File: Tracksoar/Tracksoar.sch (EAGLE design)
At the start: 35 parts, among them IC2 74AHC1G125DBV, U1 ATMEGA328P, Y1 16MHZ

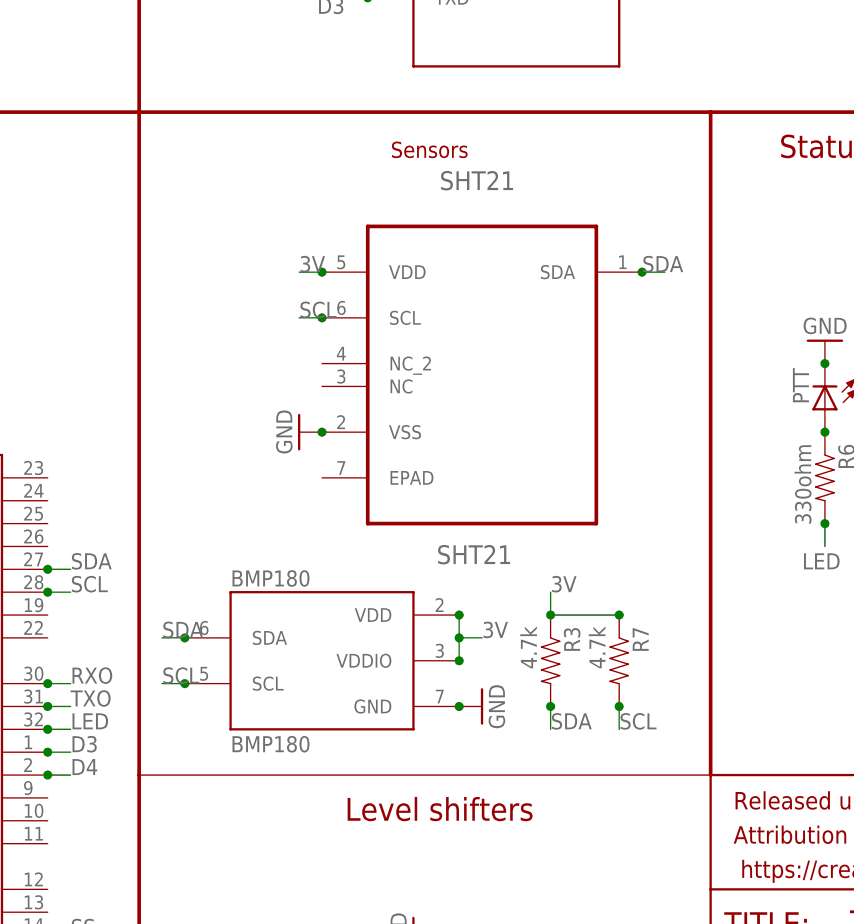
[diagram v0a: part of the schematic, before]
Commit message: Added V1.2 board
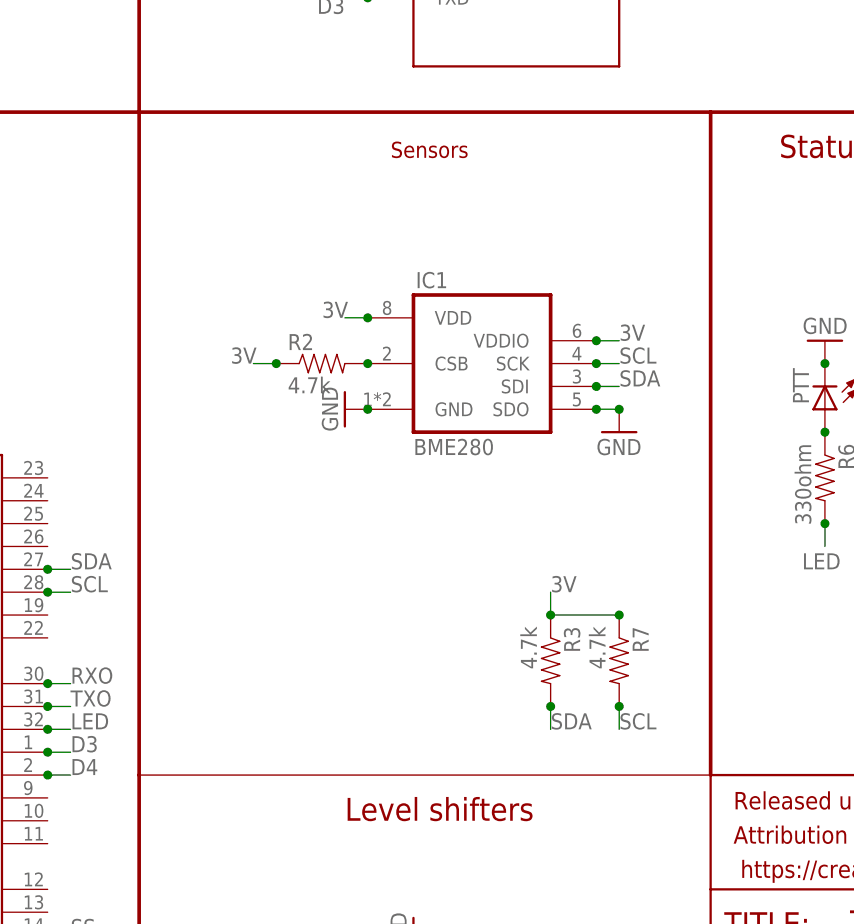
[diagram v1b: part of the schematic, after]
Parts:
- removed BMP180: BMP180, SparkFun-Sensors:BMP180
- removed SHT21: SHT21, sht21:SHT21
- added IC1: BME280, bosch-bme280:BME280
- added R2: 4.7k, SparkFun-Resistors:RESISTOR0805-RES
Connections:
- new net N$2: IC1.CSB, R2.2
- net 3V: now also IC1.VDD, IC1.VDDIO, R2.1; no longer BMP180.VDD, BMP180.VDDIO, SHT21.VDD
- net GND: now also IC1.GND, IC1.SDO; no longer BMP180.GND, SHT21.VSS
- net SCL: now also IC1.SCK; no longer BMP180.SCL, SHT21.SCL
- net SDA: now also IC1.SDI; no longer BMP180.SDA, SHT21.SDA
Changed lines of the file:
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@@
 <part name="GND3" library="SparkFun-Aesthetics" deviceset="GND" device=""/>
 <part name="GND10" library="SparkFun-Aesthetics" deviceset="GND" device=""/>
-<part name="BMP180" library="SparkFun-Sensors" deviceset="BMP180" device=""/>
-<part name="GND16" library="SparkFun-Aesthetics" deviceset="GND" device=""/>
 <part name="GND20" library="SparkFun-Aesthetics" deviceset="GND" device=""/>
 <part name="R3" library="SparkFun-Resistors" deviceset="RESISTOR" device="0805-RES" value="4.7k"/>
@@
 <part name="GND29" library="SparkFun-Aesthetics" deviceset="GND" device=""/>
 <part name="GND30" library="SparkFun-Aesthetics" deviceset="GND" device=""/>
-<part name="SHT21" library="sht21" deviceset="SHT21" device=""/>
 <part name="GPS-ANT" library="SparkFun-RF" deviceset="ANTENNA2" device="SMD3"/>
 <part name="FTDI" library="headers(2mm)" deviceset="1X7" device=""/>
@@
 <part name="U$3" library="headers(2mm)" deviceset="1X2" device=""/>
 <part name="GND5" library="SparkFun-Aesthetics" deviceset="GND" device=""/>
+<part name="IC1" library="bosch-bme280" deviceset="BME280" device=""/>
+<part name="GND6" library="SparkFun-Aesthetics" deviceset="GND" device=""/>
+<part name="R2" library="SparkFun-Resistors" deviceset="RESISTOR" device="0805-RES" value="4.7k"/>
 </parts>
 <sheets>
@@
 <instance part="GND3" gate="1" x="17.78" y="157.48"/>
 <instance part="GND10" gate="1" x="208.28" y="58.42" rot="R90"/>
-<instance part="BMP180" gate="G$1" x="104.14" y="48.26"/>
-<instance part="GND16" gate="1" x="121.92" y="43.18" rot="R90"/>
-<instance part="GND20" gate="1" x="101.6" y="73.66" rot="R270"/>
+<instance part="GND20" gate="1" x="106.68" y="76.2" rot="R270"/>
 <instance part="R3" gate="G$1" x="129.54" y="48.26" rot="R270"/>
 <instance part="R7" gate="G$1" x="137.16" y="48.26" rot="R270"/>
@@
 <instance part="GND29" gate="1" x="7.62" y="129.54"/>
 <instance part="GND30" gate="1" x="53.34" y="127"/>
-<instance part="SHT21" gate="A" x="121.92" y="83.82"/>
 <instance part="GPS-ANT" gate="G$1" x="165.1" y="165.1" rot="R90"/>
 <instance part="FTDI" gate="G$1" x="200.66" y="53.34"/>
@@
 <instance part="U$3" gate="G$1" x="40.64" y="175.26" rot="R270"/>
 <instance part="GND5" gate="1" x="38.1" y="167.64"/>
+<instance part="IC1" gate="G$1" x="121.92" y="81.28"/>
+<instance part="GND6" gate="1" x="137.16" y="73.66"/>
+<instance part="R2" gate="G$1" x="104.14" y="81.28"/>
 </instances>
 <busses>
@@
 </segment>
 <segment>
-<pinref part="BMP180" gate="G$1" pin="GND"/>
-<pinref part="GND16" gate="1" pin="GND"/>
-<junction x="119.38" y="43.18"/>
-</segment>
-<segment>
 <pinref part="LT3426" gate="G$1" pin="GND"/>
 <pinref part="GND27" gate="1" pin="GND"/>
@@
 <pinref part="GND30" gate="1" pin="GND"/>
 <junction x="53.34" y="129.54"/>
-</segment>
-<segment>
-<pinref part="SHT21" gate="A" pin="VSS"/>
-<pinref part="GND20" gate="1" pin="GND"/>
-<junction x="104.14" y="73.66"/>
 </segment>
 <segment>
@@
 <pinref part="GND5" gate="1" pin="GND"/>
 <junction x="38.1" y="170.18"/>
+</segment>
+<segment>
+<pinref part="IC1" gate="G$1" pin="GND"/>
+<pinref part="GND20" gate="1" pin="GND"/>
+<junction x="109.22" y="76.2"/>
+</segment>
+<segment>
+<pinref part="IC1" gate="G$1" pin="SDO"/>
+<pinref part="GND6" gate="1" pin="GND"/>
+<wire x1="137.16" y1="76.2" x2="134.62" y2="76.2" width="0.1524" layer="91"/>
+<junction x="134.62" y="76.2"/>
+<junction x="137.16" y="76.2"/>
 </segment>
 </net>
@@
 </segment>
 <segment>
-<pinref part="BMP180" gate="G$1" pin="VDD"/>
-<pinref part="BMP180" gate="G$1" pin="VDDIO"/>
-<wire x1="119.38" y1="53.34" x2="119.38" y2="50.8" width="0.1524" layer="91"/>
-<wire x1="119.38" y1="50.8" x2="119.38" y2="48.26" width="0.1524" layer="91"/>
-<wire x1="119.38" y1="50.8" x2="121.92" y2="50.8" width="0.1524" layer="91"/>
-<junction x="119.38" y="53.34"/>
-<junction x="119.38" y="48.26"/>
-<junction x="119.38" y="50.8"/>
-<label x="121.92" y="50.8" size="1.778" layer="95"/>
-</segment>
-<segment>
-<wire x1="104.14" y1="91.44" x2="101.6" y2="91.44" width="0.1524" layer="91"/>
-<label x="101.6" y="91.44" size="1.778" layer="95"/>
-<pinref part="SHT21" gate="A" pin="VDD"/>
-<junction x="104.14" y="91.44"/>
+<wire x1="109.22" y1="86.36" x2="106.68" y2="86.36" width="0.1524" layer="91"/>
+<label x="104.14" y="86.36" size="1.778" layer="95"/>
+<label x="137.16" y="83.82" size="1.778" layer="95"/>
+<label x="93.98" y="81.28" size="1.778" layer="95"/>
+<pinref part="IC1" gate="G$1" pin="VDD"/>
+<junction x="109.22" y="86.36"/>
 </segment>
 <segment>
@@
 <junction x="137.16" y="53.34"/>
 </segment>
+<segment>
+<wire x1="137.16" y1="83.82" x2="134.62" y2="83.82" width="0.1524" layer="91"/>
+<pinref part="IC1" gate="G$1" pin="VDDIO"/>
+<junction x="134.62" y="83.82"/>
+</segment>
+<segment>
+<wire x1="99.06" y1="81.28" x2="96.52" y2="81.28" width="0.1524" layer="91"/>
+<pinref part="R2" gate="G$1" pin="1"/>
+<junction x="99.06" y="81.28"/>
+</segment>
 </net>
 <net name="N$1" class="0">
@@
 </segment>
 <segment>
-<wire x1="142.24" y1="91.44" x2="139.7" y2="91.44" width="0.1524" layer="91"/>
-<label x="139.7" y="91.44" size="1.778" layer="95"/>
-<pinref part="SHT21" gate="A" pin="SDA"/>
-<junction x="139.7" y="91.44"/>
-</segment>
-<segment>
-<pinref part="BMP180" gate="G$1" pin="SDA"/>
-<wire x1="88.9" y1="50.8" x2="86.36" y2="50.8" width="0.1524" layer="91"/>
-<label x="86.36" y="50.8" size="1.778" layer="95"/>
-<junction x="88.9" y="50.8"/>
+<wire x1="137.16" y1="78.74" x2="134.62" y2="78.74" width="0.1524" layer="91"/>
+<label x="137.16" y="78.74" size="1.778" layer="95"/>
+<pinref part="IC1" gate="G$1" pin="SDI"/>
+<junction x="134.62" y="78.74"/>
 </segment>
 <segment>
@@
 </segment>
 <segment>
-<wire x1="104.14" y1="86.36" x2="101.6" y2="86.36" width="0.1524" layer="91"/>
-<label x="101.6" y="86.36" size="1.778" layer="95"/>
-<pinref part="SHT21" gate="A" pin="SCL"/>
-<junction x="104.14" y="86.36"/>
-</segment>
-<segment>
-<pinref part="BMP180" gate="G$1" pin="SCL"/>
-<wire x1="88.9" y1="45.72" x2="86.36" y2="45.72" width="0.1524" layer="91"/>
-<label x="86.36" y="45.72" size="1.778" layer="95"/>
-<junction x="88.9" y="45.72"/>
+<wire x1="137.16" y1="81.28" x2="134.62" y2="81.28" width="0.1524" layer="91"/>
+<label x="137.16" y="81.28" size="1.778" layer="95"/>
+<pinref part="IC1" gate="G$1" pin="SCK"/>
+<junction x="134.62" y="81.28"/>
 </segment>
 <segment>
@@
 </segment>
 </net>
+<net name="N$2" class="0">
+<segment>
+<pinref part="IC1" gate="G$1" pin="CSB"/>
+<pinref part="R2" gate="G$1" pin="2"/>
+<junction x="109.22" y="81.28"/>
+</segment>
+</net>
 </nets>
 </sheet>
@@
 </schematic>
 </drawing>
+<compatibility>
+<note version="6.3" minversion="6.2.2" severity="warning">
+Since Version 6.2.2 text objects can contain more than one line,
+which will not be processed correctly with this version.
+</note>
+</compatibility>
 </eagle>
